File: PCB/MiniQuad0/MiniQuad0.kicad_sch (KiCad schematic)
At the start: 15 parts, among them J1 R8EF_Radio, J2 MPU6500, J3 ESC_A, J4 ESC_B, J5 ESC_C, J6 ESC_D, J7 POWER, J8 VBAT, J9 RADIO_SIG, Q1 2N2219, U2 XIAO-RP2350-SMD

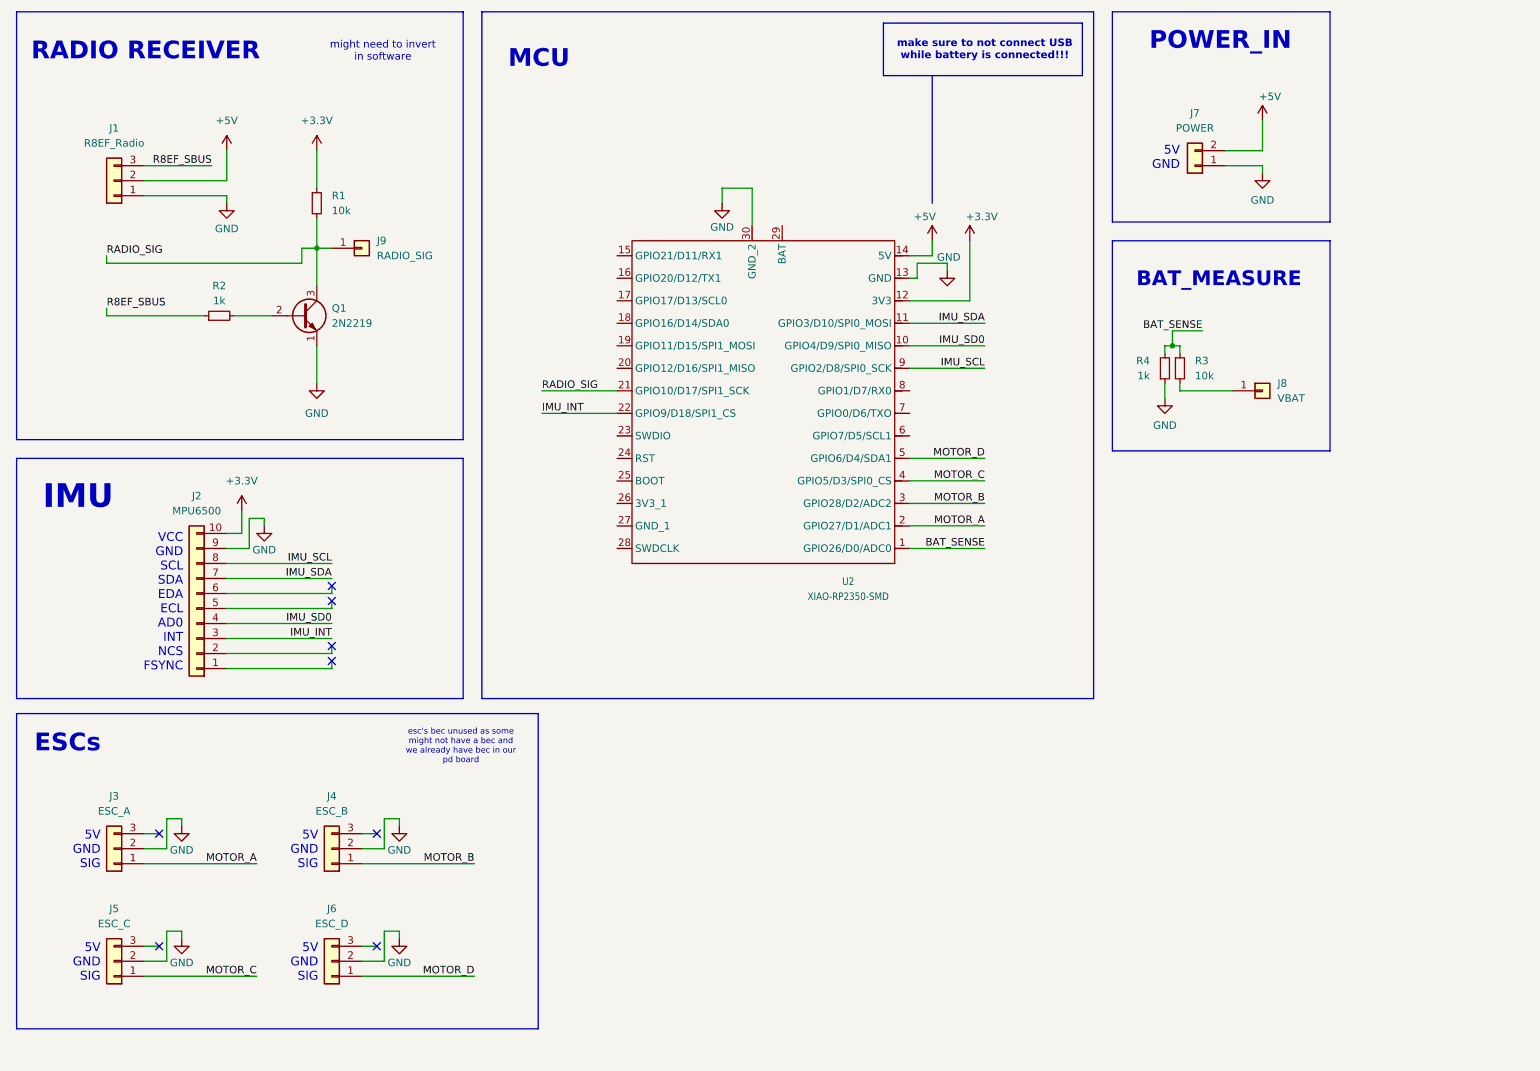
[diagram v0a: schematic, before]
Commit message: schematics update, pcb layout r2
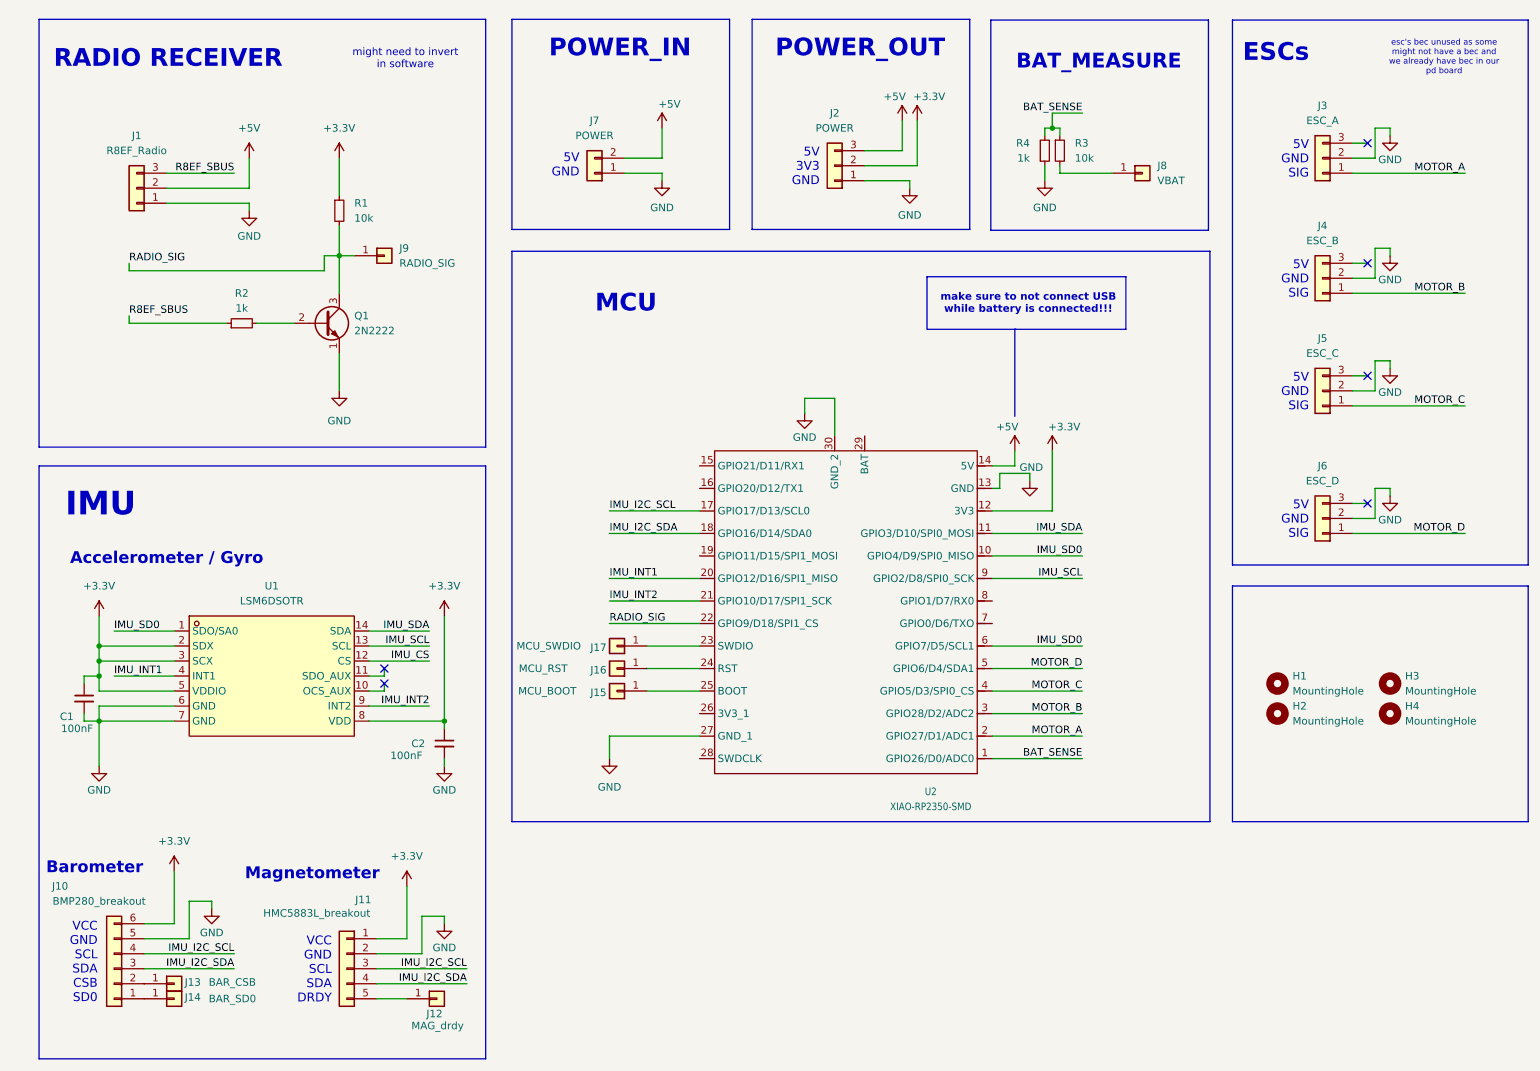
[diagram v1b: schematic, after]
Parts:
- removed J2: MPU6500, Connector_PinHeader_2.54mm:PinHeader_1x10_P2.54mm_Vertical, symbol Connector_Generic:Conn_01x10
- added C1, C2: 100nF, Capacitor_SMD:C_0603_1608Metric_Pad1.08x0.95mm_HandSolder, symbol Device:C_Small
- added H1, H2, H3, H4: MountingHole, MountingHole:MountingHole_3mm, symbol Mechanical:MountingHole
- added J10: BMP280_breakout, Connector_PinHeader_2.54mm:PinHeader_1x06_P2.54mm_Vertical, symbol Connector_Generic:Conn_01x06
- added J11: HMC5883L_breakout, Connector_PinHeader_2.54mm:PinHeader_1x05_P2.54mm_Vertical, symbol Connector_Generic:Conn_01x05
- added J12: MAG_drdy, TestPoint:TestPoint_Pad_D1.0mm, symbol Connector_Generic:Conn_01x01
- added J13: BAR_CSB, TestPoint:TestPoint_Pad_D1.0mm, symbol Connector_Generic:Conn_01x01
- added J14: BAR_SD0, TestPoint:TestPoint_Pad_D1.0mm, symbol Connector_Generic:Conn_01x01
- added J15: MCU_BOOT, TestPoint:TestPoint_Pad_D1.0mm, symbol Connector_Generic:Conn_01x01
- added J16: MCU_RST, TestPoint:TestPoint_Pad_D1.0mm, symbol Connector_Generic:Conn_01x01
- added J17: MCU_SWDIO, TestPoint:TestPoint_Pad_D1.0mm, symbol Connector_Generic:Conn_01x01
- added J2: POWER, Connector_PinHeader_2.54mm:PinHeader_1x03_P2.54mm_Vertical, symbol Connector_Generic:Conn_01x03
- added U1: LSM6DSOTR, easyeda2kicad:LGA-14_L3.0-W2.5-P0.50-TL, symbol easyeda2kicad:LSM6DSOTR
- J9: footprint Connector_PinHeader_2.54mm:PinHeader_1x01_P2.54mm_Vertical -> TestPoint:TestPoint_Pad_D1.0mm
- Q1: value 2N2219 -> 2N2222; footprint Connector_PinHeader_2.54mm:PinHeader_1x03_P2.54mm_Vertical -> Package_TO_SOT_SMD:TSOT-23_HandSoldering
- R1, R2, R3, R4: footprint Connector_PinHeader_2.54mm:PinHeader_1x02_P2.54mm_Vertical -> Resistor_SMD:R_1206_3216Metric_Pad1.30x1.75mm_HandSolder
- U2: footprint Seeed Studio XIAO Series Library:XIAO-RP2350-DIP -> Seeed Studio XIAO Series Library:XIAO-RP2350-SMD
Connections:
- net IMU_INT is gone; now on net RADIO_SIG: U2.22 (GPIO9/D18/SPI1_CS)
- net +3.3V: now also C1.1, C2.1, J10.6 (Pin_6), J11.1 (Pin_1), J2.2 (Pin_2), U1.2 (SDX), U1.3 (SCX), U1.5 (VDDIO), U1.8 (VDD)
- net +5V: now also J2.3 (Pin_3)
- net GND: now also U2.27 (GND_1), C1.2, C2.2, J10.5 (Pin_5), J11.2 (Pin_2), J2.1 (Pin_1), U1.6 (GND), U1.7 (GND)
- net IMU_SCL: now also U1.13 (SCL)
- net IMU_SD0: now also U2.6 (GPIO7/D5/SCL1), U1.1 (SDO/SA0)
- net IMU_SDA: now also U1.14 (SDA)
- net RADIO_SIG: no longer U2.21 (GPIO10/D17/SPI1_SCK)
- net IMU_I2C_SCL: now reaches U2.17 (GPIO17/D13/SCL0)
- net IMU_I2C_SCL: now also J10.4 (Pin_4), J11.3 (Pin_3)
- net IMU_I2C_SDA: now reaches U2.18 (GPIO16/D14/SDA0)
- net IMU_I2C_SDA: now also J10.3 (Pin_3), J11.4 (Pin_4)
- net IMU_INT1: now reaches U2.20 (GPIO12/D16/SPI1_MISO)
- net IMU_INT1: now also U1.4 (INT1)
- net at U2.23 (SWDIO): now also J17.1 (Pin_1)
- net at U2.24 (RST): now also J16.1 (Pin_1)
- net at U2.25 (BOOT): now also J15.1 (Pin_1)
- new net: J11.5 (Pin_5), J12.1 (Pin_1)
- new net: J10.1 (Pin_1), J14.1 (Pin_1)
- new net: J10.2 (Pin_2), J13.1 (Pin_1)
- new net IMU_CS: U1.12 (CS)
- new net IMU_INT2: U1.9 (INT2), U2.21 (GPIO10/D17/SPI1_SCK)
- no-connect marks 8 -> 6
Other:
- note added: "5V 3V3 GND"
- note added: "Accelerometer / Gyro"
- note added: "Barometer"
- note added: "Magnetometer"
- note added: "POWER_OUT"
- note added: "VCC GND SCL SDA CSB SD0"
- note added: "VCC GND SCL SDA DRDY"
- note removed: "VCC GND SCL SDA EDA ECL AD0 INT NCS FSYNC"
- moved on the sheet: J1, J3, J4, J5, J6, J7, J8, J9, Q1, R1, R2, R3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
